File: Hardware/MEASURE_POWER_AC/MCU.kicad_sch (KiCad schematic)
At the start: 30 parts, among them J1 Conn_01x04_Pin, SW1 RESET, U1 STM32F103C8T6, Y1 Crystal_8MHz_SMD-4PIN

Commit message: Update BOM
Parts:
- SW1: Supply URL (none) -> https://www.thegioiic.com/nut-nhan-3x4mm-cao-2-5mm-2-chan-s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; Suppy URL https://www.thegioiic.com/nut-nhan-3x4mm-cao-2-5mm-2-chan-s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 -> (none)
- U1: Supply name (none) -> Thegioiic; Supply name  Thegioiic -> (none)
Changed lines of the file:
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@@
 			)
 		)
-		(property "Suppy URL" "https://www.thegioiic.com/nut-nhan-3x4mm-cao-2-5mm-2-chan-smd"
+		(property "Suppy URL" ""
 			(at 245.11 106.426 0)
+			(effects
+				(font
+					(size 1.27 1.27)
+				)
+				(hide yes)
+			)
+		)
+		(property "Supply URL" "https://www.thegioiic.com/nut-nhan-3x4mm-cao-2-5mm-2-chan-smd"
+			(at 251.46 105.41 0)
 			(effects
 				(font
@@
 			)
 		)
-		(property "Supply name " "Thegioiic"
+		(property "Supply name " ""
 			(at 96.52 110.49 0)
 			(effects
@@
 		)
 		(property "Supply URL" "https://www.thegioiic.com/stm32f103c8t6-32-bit-arm-cortex-m3-microcontroller-72mhz-64kb-flash-48-lqfp"
+			(at 96.52 110.49 0)
+			(effects
+				(font
+					(size 1.27 1.27)
+				)
+				(hide yes)
+			)
+		)
+		(property "Supply name" "Thegioiic"
 			(at 96.52 110.49 0)
 			(effects
@@
 			)
 		)
-		(property "Supply name " "Thegioiic"
+		(property "Supply name " ""
 			(at 186.69 45.72 0)
 			(effects
@@
 			(at 186.69 45.72 0)
 			(effects
+				(font
+					(size 1.27 1.27)
+				)
+				(hide yes)
+			)
+		)
+		(property "Supply name" "Thegioiic"
+			(at 186.69 45.72 0)
+			(effects

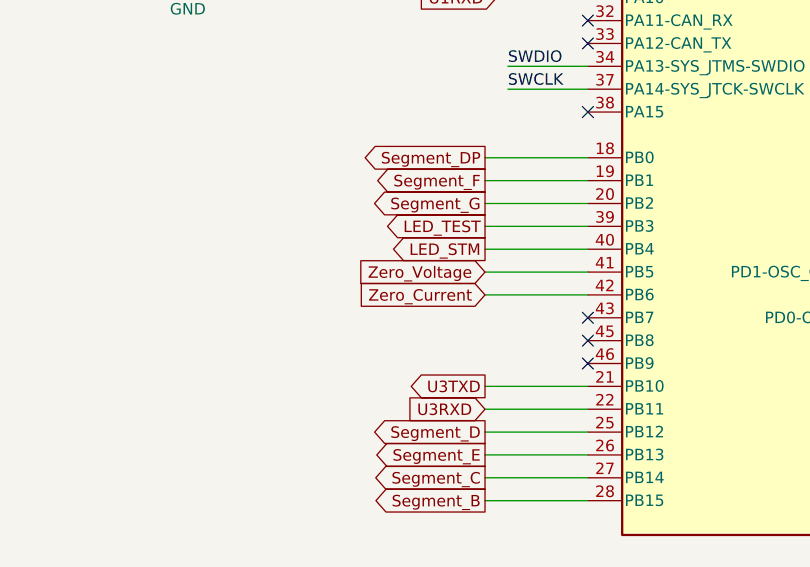
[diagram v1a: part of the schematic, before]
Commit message: Update
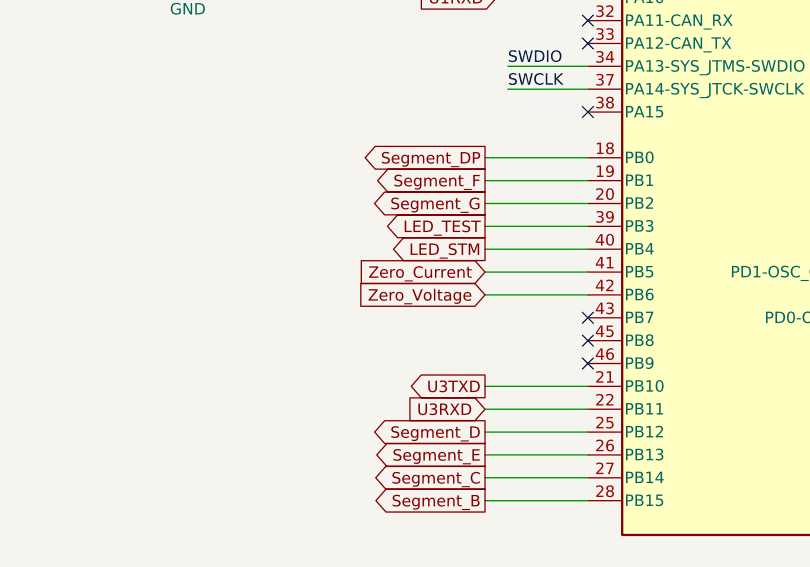
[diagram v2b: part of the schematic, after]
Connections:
- net Zero_Current: now also U1.41 (PB5); no longer U1.42 (PB6)
- net Zero_Voltage: now also U1.42 (PB6); no longer U1.41 (PB5)
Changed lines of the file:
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@@
 		)
 	)
-	(global_label "Zero_Voltage"
+	(global_label "Zero_Current"
 		(shape input)
 		(at 81.28 81.28 180)
@@
 		)
 		(property "Intersheetrefs" "${INTERSHEET_REFS}"
-			(at 66.0788 81.28 0)
+			(at 66.1392 81.28 0)
 			(effects
 				(font
@@
 		)
 	)
-	(global_label "Zero_Current"
+	(global_label "Zero_Voltage"
 		(shape input)
 		(at 81.28 83.82 180)
@@
 		)
 		(property "Intersheetrefs" "${INTERSHEET_REFS}"
-			(at 66.1392 83.82 0)
+			(at 66.0788 83.82 0)
 			(effects
 				(font
